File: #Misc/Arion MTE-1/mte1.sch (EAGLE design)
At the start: 21 parts

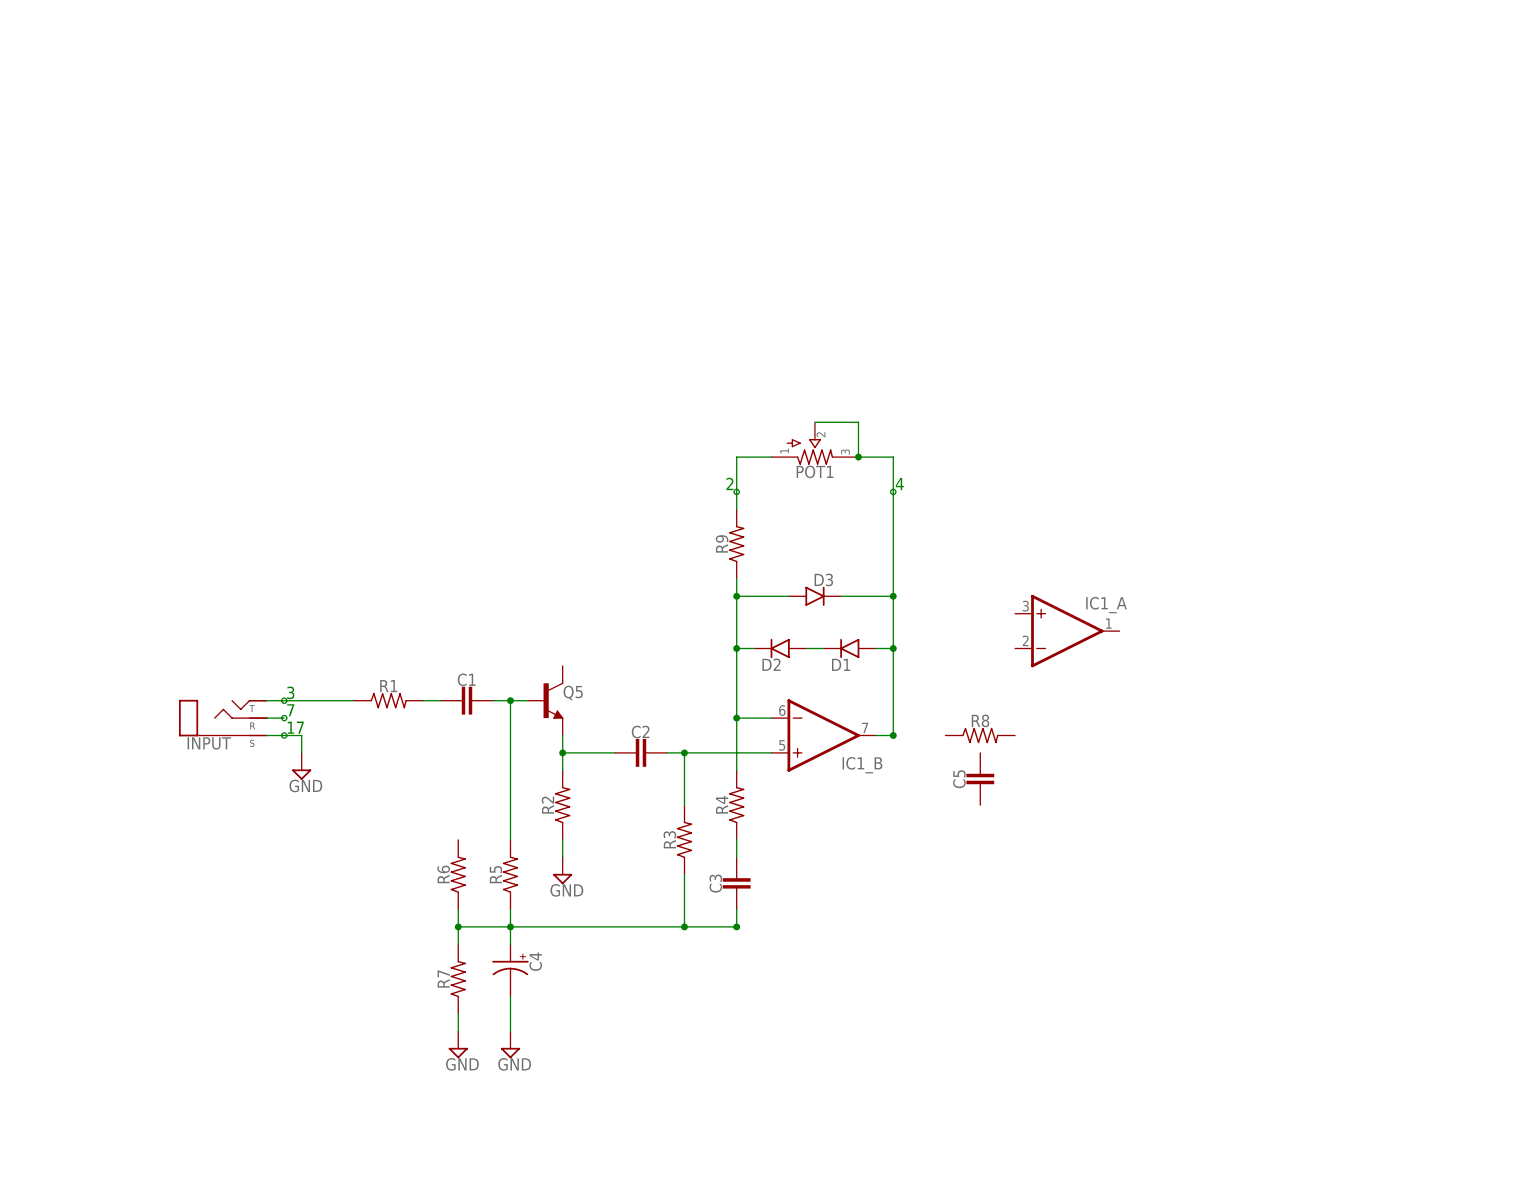
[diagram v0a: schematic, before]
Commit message: 20171111
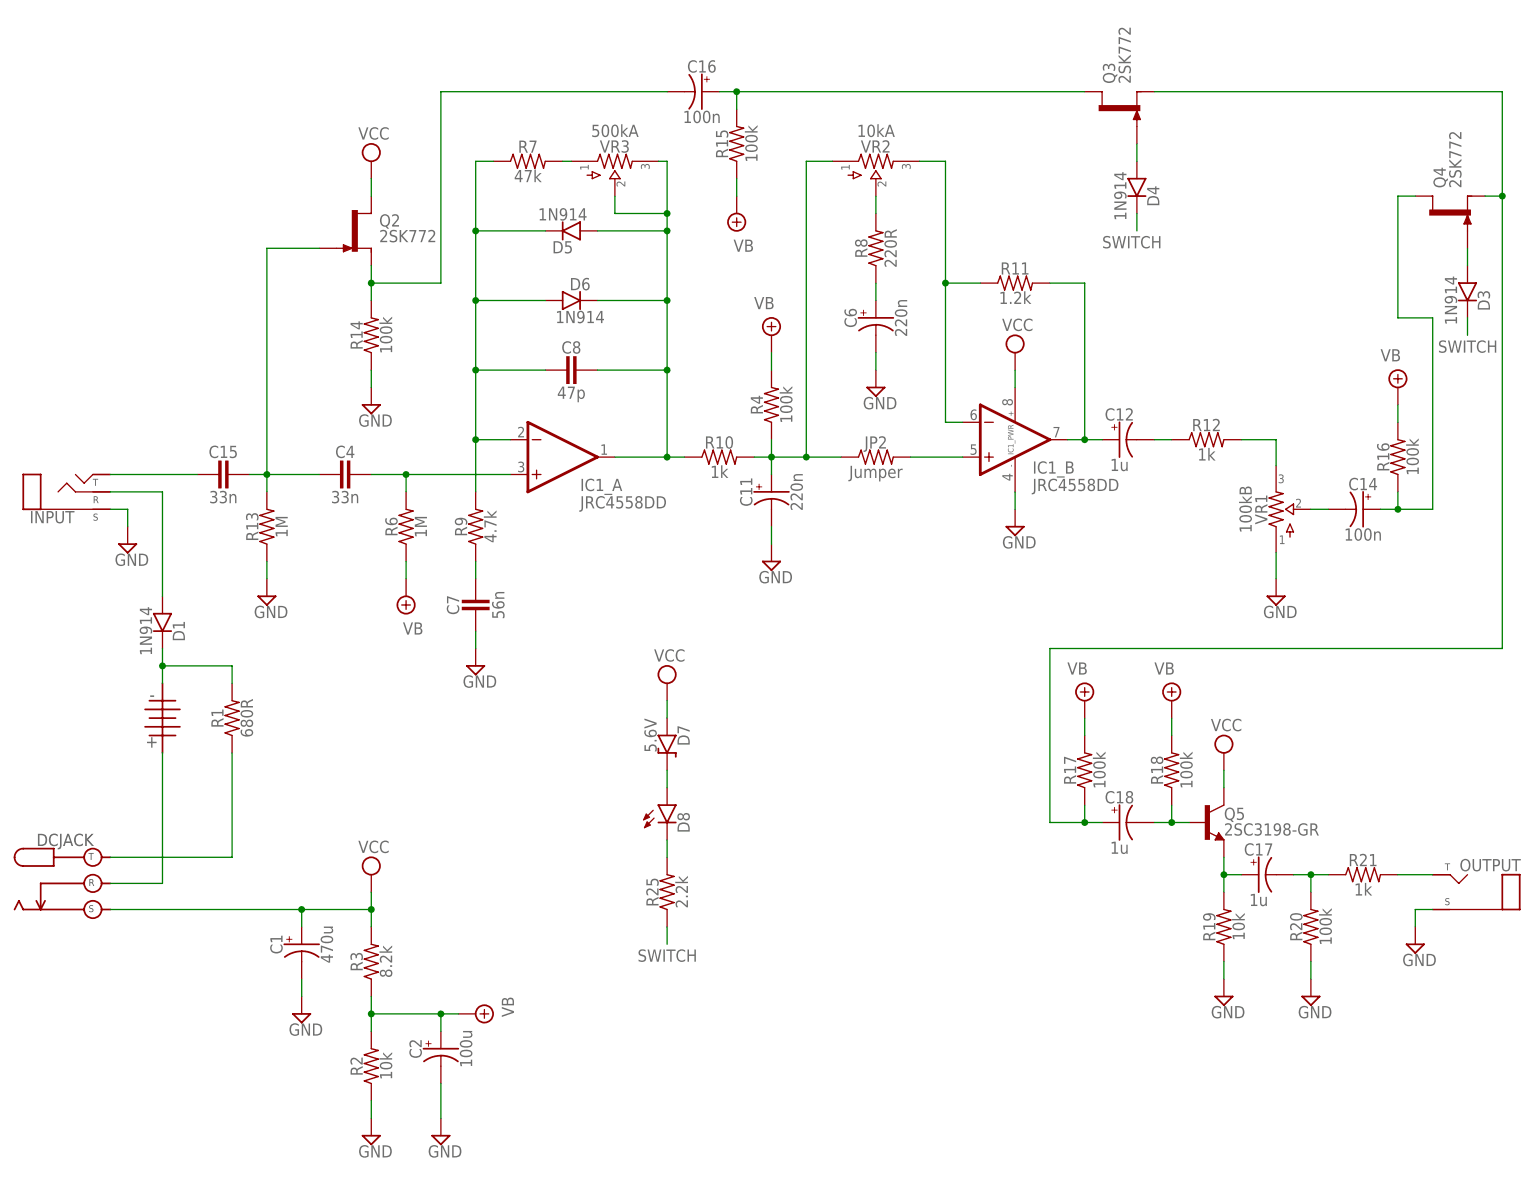
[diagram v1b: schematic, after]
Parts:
- removed C3, C5: (no value), pedals-capacitors-film:CER/FILMBOX.1
- removed D2: (no value), pedals-diodes:DO35.2
- removed POT1: (no value), pedals-potentiometers:POTS16MM
- removed R5: (no value), pedals-resistors:R_.3B
- added 1101: BATTERY, pedals-jacks:BATTERY
- added C11, C6: 220n, pedals-capacitors-elec:0400
- added C12, C17, C18: 1u, pedals-capacitors-elec:0400
- added C14, C16: 100n, pedals-capacitors-elec:0400
- added C15: 33n, pedals-capacitors-film:CER/FILMBOX.1
- added C7: 56n, pedals-capacitors-film:CER/FILMBOX.1
- added C8: 47p, pedals-capacitors-film:CER/FILMBOX.1
- added D4, D5, D6: 1N914, pedals-diodes:DO35.2
- added D7: 5.6V, pedals-diodes:ZENER.2
- added D8: LED, pedals-diodes:LED
- added DCJACK: DCJACK, pedals-jacks:DC_KOBICONN
- added JP2: Jumper, pedals-resistors:R_.3B
- added OUTPUT: (no value), pedals-jacks:MONO
- added Q2, Q3, Q4: 2SK772, pedals-transistors:2N5457
- added R10, R12, R21: 1k, pedals-resistors:R_.3B
- added R11: 1.2k, pedals-resistors:R_.3B
- added R13: 1M, pedals-resistors:R_.3B
- added R14, R15, R16, R17, R18, R20: 100k, pedals-resistors:R_.3B
- added R19: 10k, pedals-resistors:R_.3B
- added R25: 2.2k, pedals-resistors:R_.3B
- added VR1: 100kB, pedals-potentiometers:POTS16MM
- added VR2: 10kA, pedals-potentiometers:POTS16MM
- added VR3: 500kA, pedals-potentiometers:POTS16MM
- C1: value (none) -> 470u; device pedals-capacitors-film:CER/FILMBOX.1 -> pedals-capacitors-elec:0400
- C2: value (none) -> 100u; device pedals-capacitors-film:CER/FILMBOX.1 -> pedals-capacitors-elec:0400
- C4: value (none) -> 33n; device pedals-capacitors-elec:0400 -> pedals-capacitors-film:CER/FILMBOX.1
- D1, D3: value (none) -> 1N914
- IC1: value (none) -> JRC4558DD
- INPUT: value (none) -> INPUT; device pedals-jacks:STEREO3PADS -> pedals-jacks:STEREO
- Q5: value (none) -> 2SC3198-GR; device pedals-transistors:2SC828A -> pedals-transistors:2N3904
- R1: value (none) -> 680R
- R2: value (none) -> 10k
- R3: value (none) -> 8.2k
- R4: value (none) -> 100k
- R6: value (none) -> 1M
- R7: value (none) -> 47k
- R8: value (none) -> 220R
- R9: value (none) -> 4.7k
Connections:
- new net DCJACK: DCJACK.T, R1.1
- new net N$13: C4.1, IC1_A.+IN, R6.2
- new net N$14: IC1_B.-IN, R11.1, VR2.3
- new net N$15: C12.+, IC1_B.OUT, R11.2
- new net N$16: R8.2, VR2.2
- new net N$17: C6.+, R8.1
- new net N$18: C12.-, R12.1
- new net N$19: R12.2, VR1.3
- new net N$20: D7.C, D8.A
- new net N$21: C14.+, Q4.D, R16.1
- new net N$22: C16.-, Q2.S, R14.2
- new net N$23: C16.+, Q3.D, R15.2
- new net N$24: D4.A, Q3.G
- new net N$25: C18.+, Q3.S, Q4.S, R17.1
- new net N$26: D3.A, Q4.G
- new net N$27: C18.-, Q5.B, R18.1
- new net N$28: C17.+, Q5.E, R19.2
- new net N$29: C17.-, R20.2, R21.1
- new net N$30: OUTPUT.TIP, R21.2
- new net N$31: D8.C, R25.2
- new net SWITCH: D4.C
- new net VB: C2.+, R15.1, R16.2, R17.2, R18.2, R2.2, R3.1, R4.2, R6.1
- new net VCC: C1.+, D7.A, DCJACK.S, IC1_PWR.V+, Q2.D, Q5.C, R3.2
- net GND: now also C1.-, C11.-, C2.-, C6.-, C7.2, IC1_PWR.V-, OUTPUT.SLEEVE, R13.1, R14.1, R19.1, R20.1, VR1.1; no longer C4.-, R7.1
- net N$1: now also D1.A, INPUT.R; no longer INPUT.T, R1.1
- net N$10: now also IC1_B.+IN, JP2.2; no longer D1.C, D2.A
- net N$11: now also C15.2, INPUT.T; no longer D1.A, D3.C, IC1_B.OUT, POT1.2, POT1.3
- net N$12: now also C15.1, C4.2, Q2.G, R13.2; no longer POT1.1, R9.2
- net N$2: now also C14.-, VR1.2; no longer INPUT.R
- net N$3: now also 1101.P$1, DCJACK.R; no longer C1.2, R1.2
- net N$4: now also 1101.P$2, D1.C, R1.2; no longer C1.1, Q5.B, R5.2
- net N$5: now also C7.1; no longer D2.C, D3.A, IC1_B.-IN, R4.2
- net N$6: now also C11.+, JP2.1, R10.2, R4.1, VR2.1; no longer C3.2, C4.+, R3.1, R5.1, R6.1, R7.2
- net N$7: now also C8.2, D5.C, D6.A, IC1_A.-IN, R7.1, R9.2; no longer C2.2, Q5.E, R2.2
- net N$8: now also R7.2, VR3.1; no longer C2.1, IC1_B.+IN, R3.2
- net N$9: now also C8.1, D5.A, D6.C, IC1_A.OUT, R10.1, VR3.2, VR3.3; no longer C3.1, R4.1
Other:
- note removed: "17"
- note removed: "2"
- note removed: "3"
- note removed: "4"
- note removed: "7"
- moved on the sheet: D1, D3, IC1_A, IC1_B, INPUT, R1, R2, R3, R4, R6, R7, R8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
